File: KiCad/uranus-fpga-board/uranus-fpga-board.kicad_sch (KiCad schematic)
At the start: 0 parts

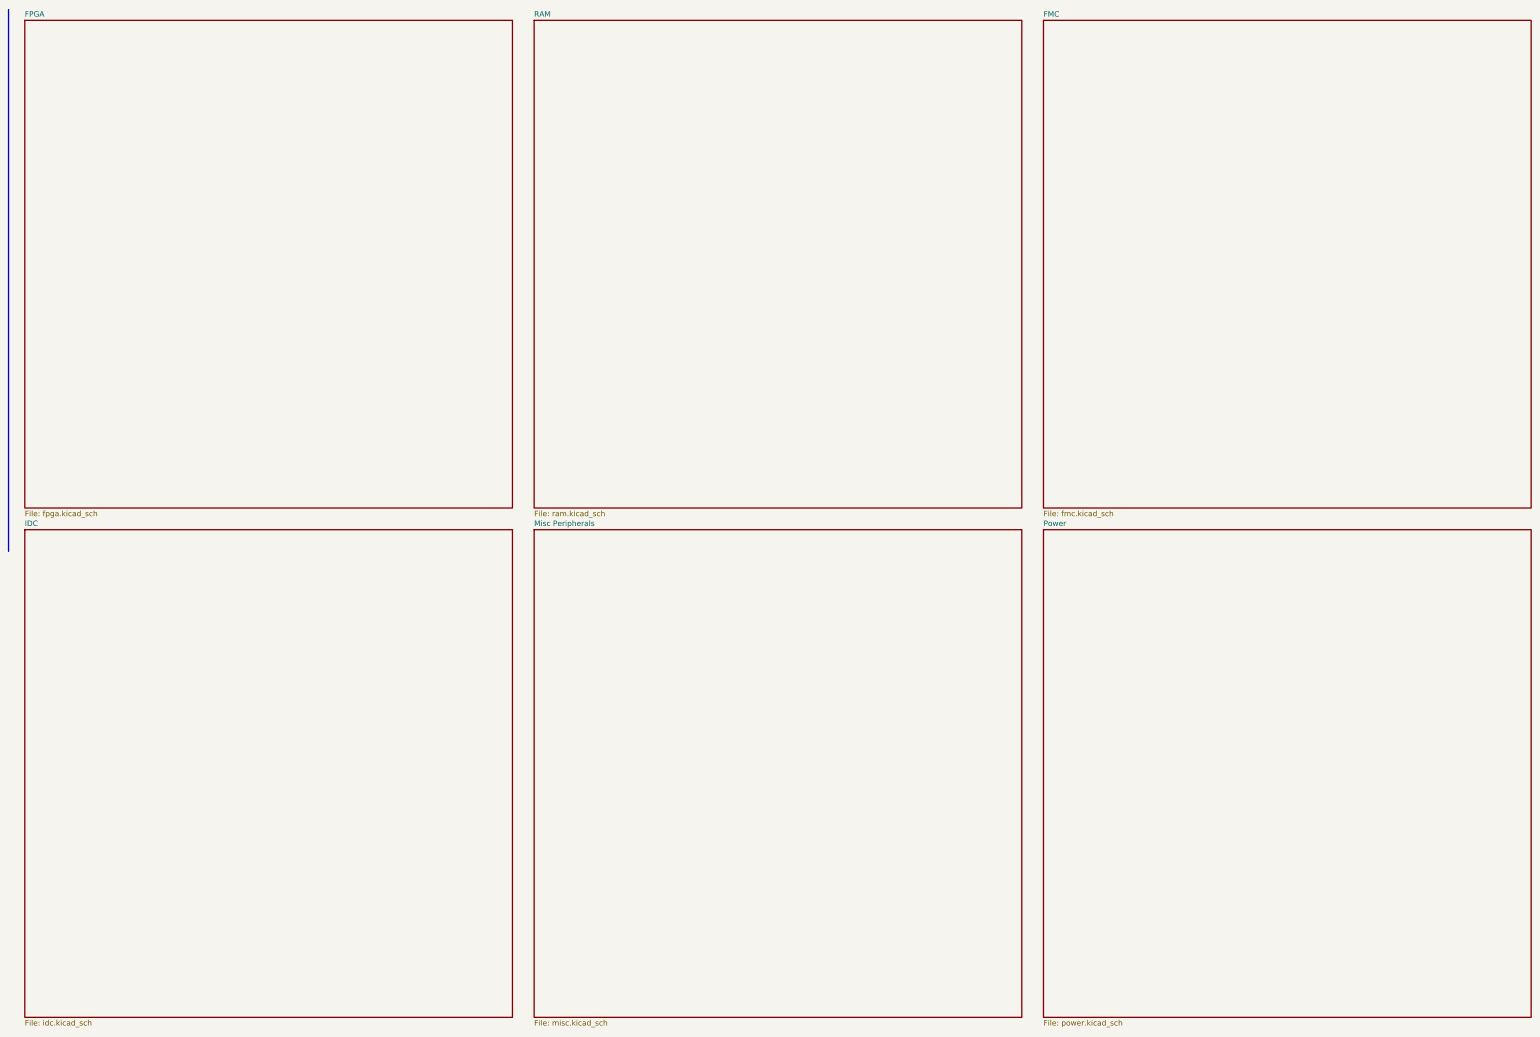
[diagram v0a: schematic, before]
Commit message: big things happening in schematic quality
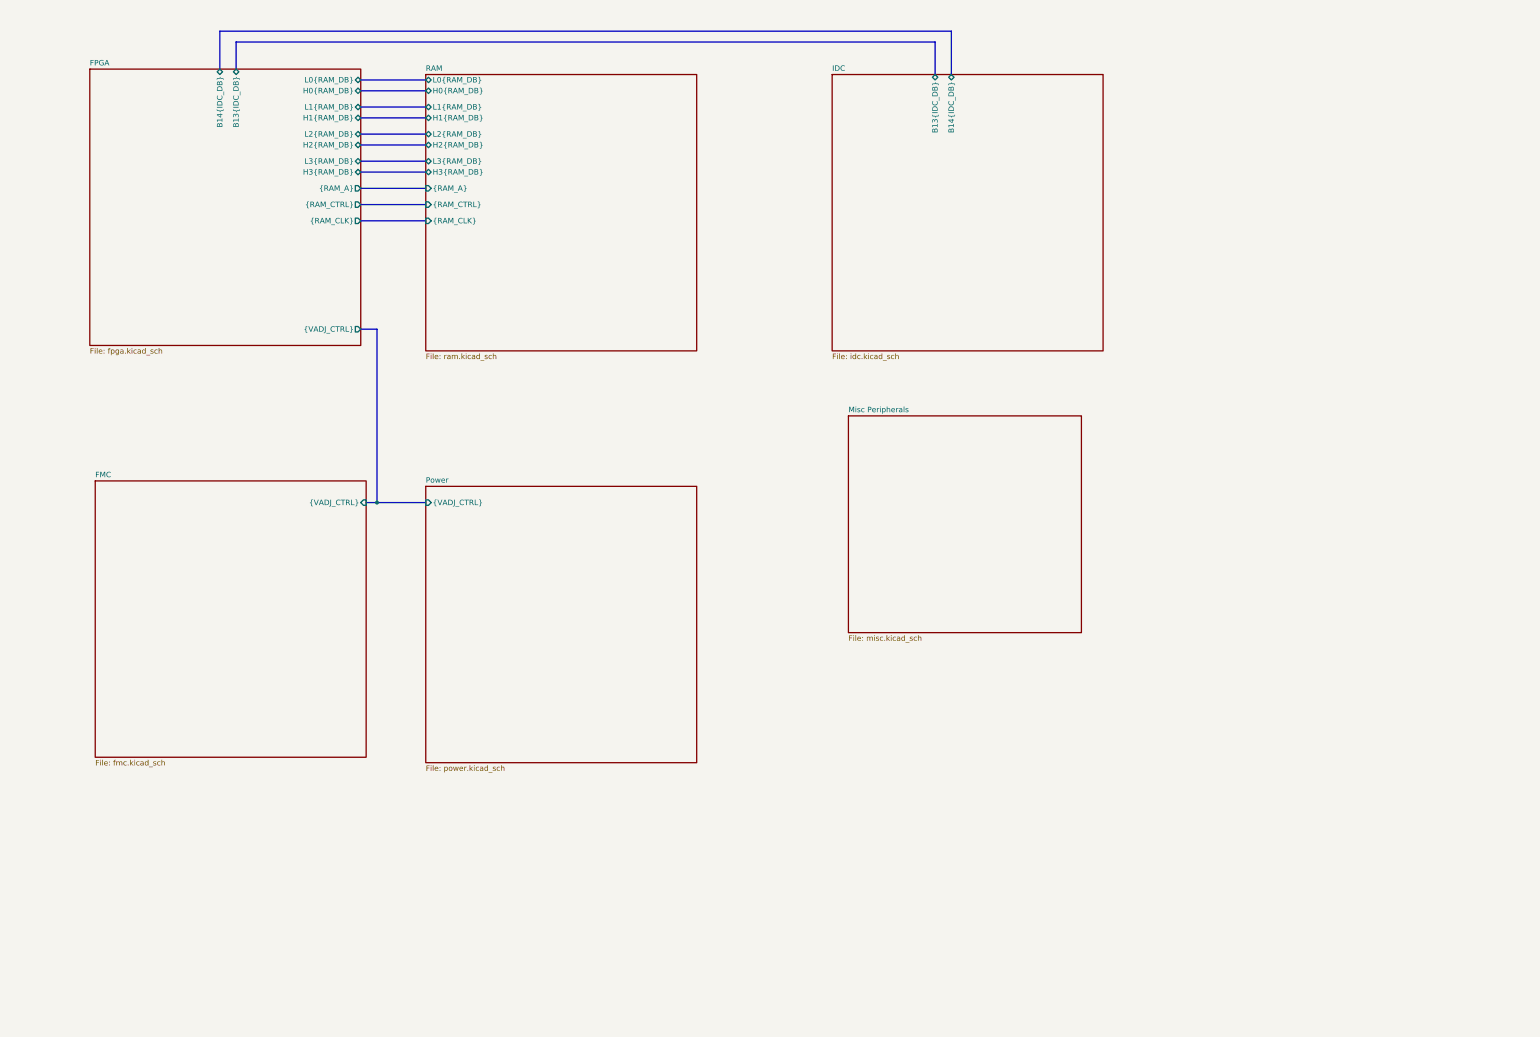
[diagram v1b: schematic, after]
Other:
- sheet FMC ports: added {VADJ_CTRL}; removed none
- sheet FPGA ports: added B13{IDC_DB}, B14{IDC_DB}, H0{RAM_DB}, H1{RAM_DB}, H2{RAM_DB}, H3{RAM_DB}, L0{RAM_DB}, L1{RAM_DB}, L2{RAM_DB}, L3{RAM_DB}, {RAM_A}, {RAM_CLK}, {RAM_CTRL}, {VADJ_CTRL}; removed none
- sheet IDC ports: added B13{IDC_DB}, B14{IDC_DB}; removed none
- sheet Power ports: added {VADJ_CTRL}; removed none
- sheet RAM ports: added H0{RAM_DB}, H1{RAM_DB}, H2{RAM_DB}, H3{RAM_DB}, L0{RAM_DB}, L1{RAM_DB}, L2{RAM_DB}, L3{RAM_DB}, {RAM_A}, {RAM_CLK}, {RAM_CTRL}; removed none

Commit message: Big things have mostly happened in schematic quality
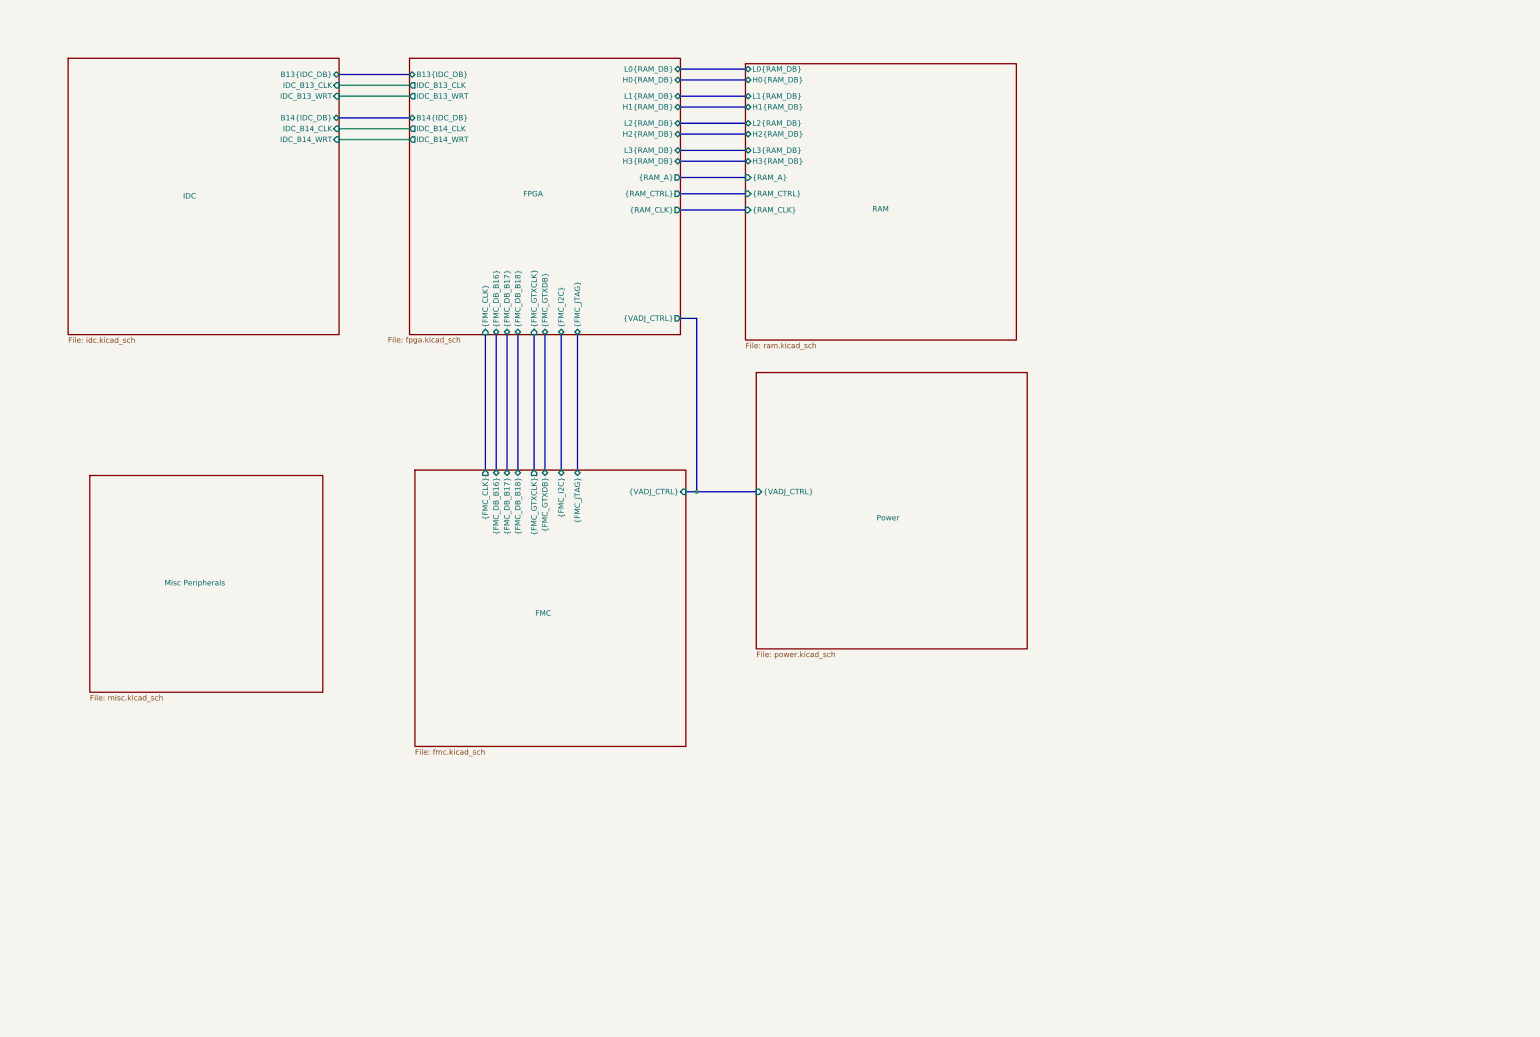
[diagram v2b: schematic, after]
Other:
- sheet FMC ports: added {FMC_CLK}, {FMC_DB_B16}, {FMC_DB_B17}, {FMC_DB_B18}, {FMC_GTXCLK}, {FMC_GTXDB}, {FMC_I2C}, {FMC_JTAG}; removed none
- sheet FPGA ports: added IDC_B13_CLK, IDC_B13_WRT, IDC_B14_CLK, IDC_B14_WRT, {FMC_CLK}, {FMC_DB_B16}, {FMC_DB_B17}, {FMC_DB_B18}, {FMC_GTXCLK}, {FMC_GTXDB}, {FMC_I2C}, {FMC_JTAG}; removed none
- sheet IDC ports: added IDC_B13_CLK, IDC_B13_WRT, IDC_B14_CLK, IDC_B14_WRT; removed none
